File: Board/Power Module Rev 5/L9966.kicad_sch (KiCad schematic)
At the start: 32 parts, among them U2 L9966CB-TR

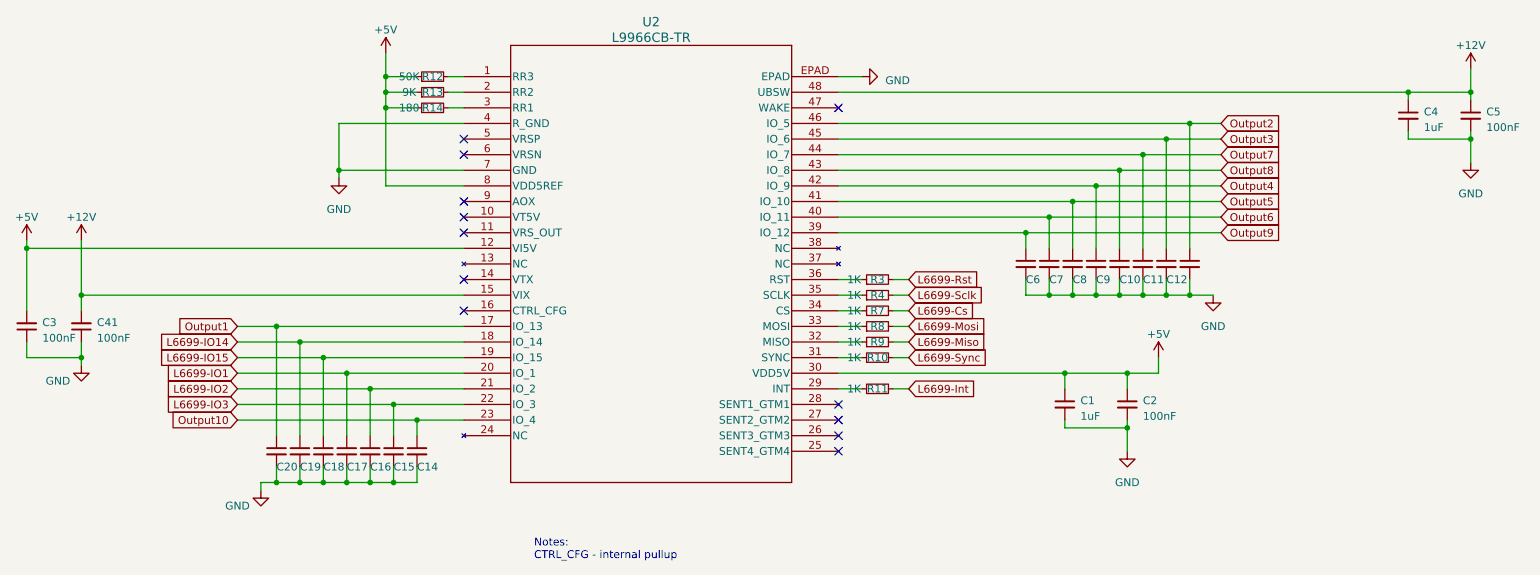
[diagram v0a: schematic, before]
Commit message: Board Update
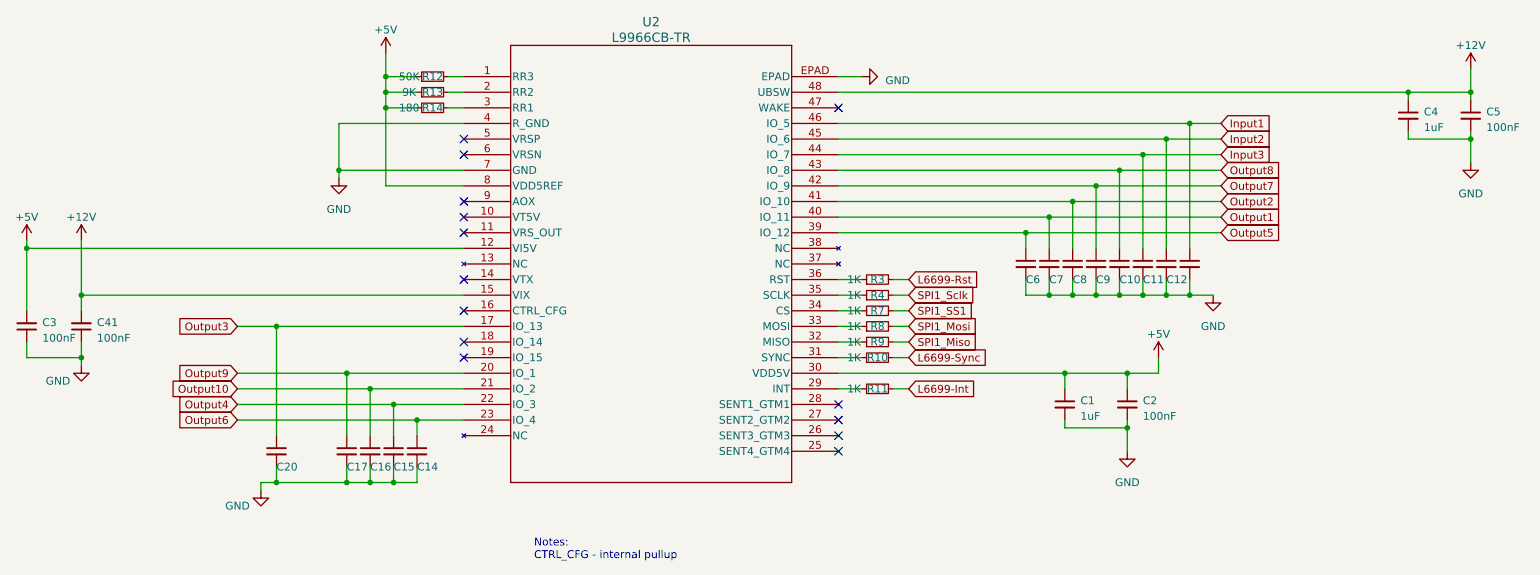
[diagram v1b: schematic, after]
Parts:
- removed C18, C19: 6.8nF, Capacitor_SMD:C_0603_1608Metric_Pad1.08x0.95mm_HandSolder, symbol Device:C_Small
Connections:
- net L6699-IO1 is gone; now on net Output9: C17.1, U2.20 (IO_1)
- net L6699-IO2 is gone; now on net Output10: C16.1, U2.21 (IO_2)
- net L6699-IO3 is gone; now on net Output4: C15.1, U2.22 (IO_3)
- net Output1: now also C7.1, U2.40 (IO_11); no longer C20.1, U2.17 (IO_13)
- net Output10: no longer C14.1, U2.23 (IO_4)
- net Output2: now also C8.1, U2.41 (IO_10); no longer C13.1, U2.46 (IO_5)
- net Output3: now also C20.1, U2.17 (IO_13); no longer C12.1, U2.45 (IO_6)
- net Output4: no longer C9.1, U2.42 (IO_9)
- net Output5: now also C6.1, U2.39 (IO_12); no longer C8.1, U2.41 (IO_10)
- net Output6: now also C14.1, U2.23 (IO_4); no longer C7.1, U2.40 (IO_11)
- net Output7: now also C9.1, U2.42 (IO_9); no longer C11.1, U2.44 (IO_7)
- net Output9: no longer C6.1, U2.39 (IO_12)
- net L6699-Cs renamed SPI1_SS1
- net L6699-IO14: no longer names the net of U2.18 (IO_14)
- net L6699-IO15: no longer names the net of U2.19 (IO_15)
- net L6699-Miso renamed SPI1_Miso
- net L6699-Mosi renamed SPI1_Mosi
- net L6699-Sclk renamed SPI1_Sclk
- new net Input1: C13.1, U2.46 (IO_5)
- new net Input2: C12.1, U2.45 (IO_6)
- new net Input3: C11.1, U2.44 (IO_7)
- no-connect marks 12 -> 14

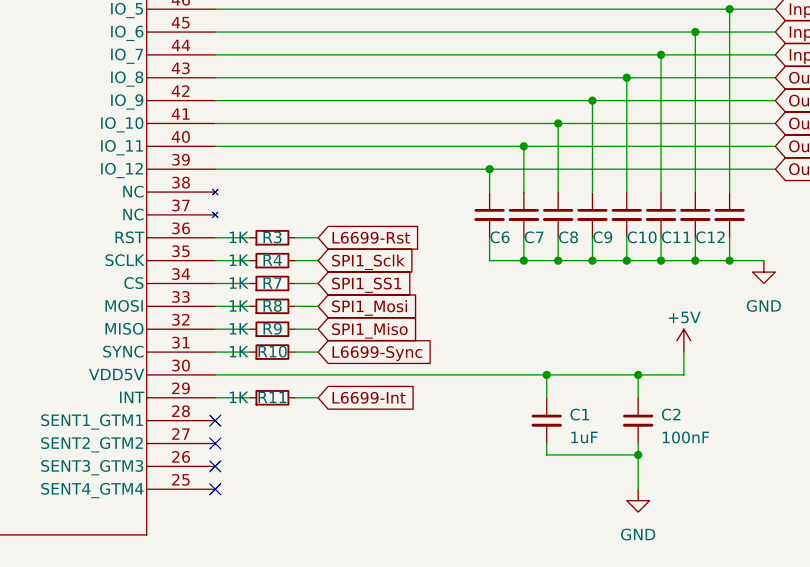
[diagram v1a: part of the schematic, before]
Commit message: Update config and renames on schematic
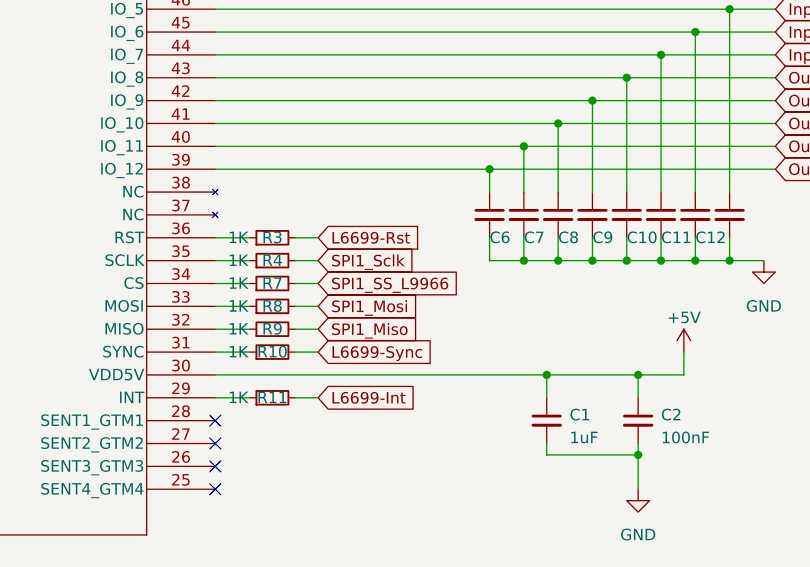
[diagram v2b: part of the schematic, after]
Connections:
- net SPI1_SS1 renamed SPI1_SS_L9966
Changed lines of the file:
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@@
     )
   )
-  (global_label "SPI1_SS1" (shape input) (at 167.64 101.6 0) (fields_autoplaced)
+  (global_label "SPI1_SS_L9966" (shape input) (at 167.64 101.6 0) (fields_autoplaced)
     (effects (font (size 1.27 1.27)) (justify left))
-    (property "Intersheetrefs" "${INTERSHEET_REFS}" (at 179.4357 101.6 0)
+    (property "Intersheetrefs" "${INTERSHEET_REFS}" (at 185.0599 101.6 0)
       (effects (font (size 1.27 1.27)) (justify left) hide)
     )
